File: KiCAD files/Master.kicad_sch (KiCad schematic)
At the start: 24 parts, among them SW1 EG1271A, SW2 EG1271A, SW3 EG1271A, SW4 EG1271A, U4 NUCLEO64-F446RE

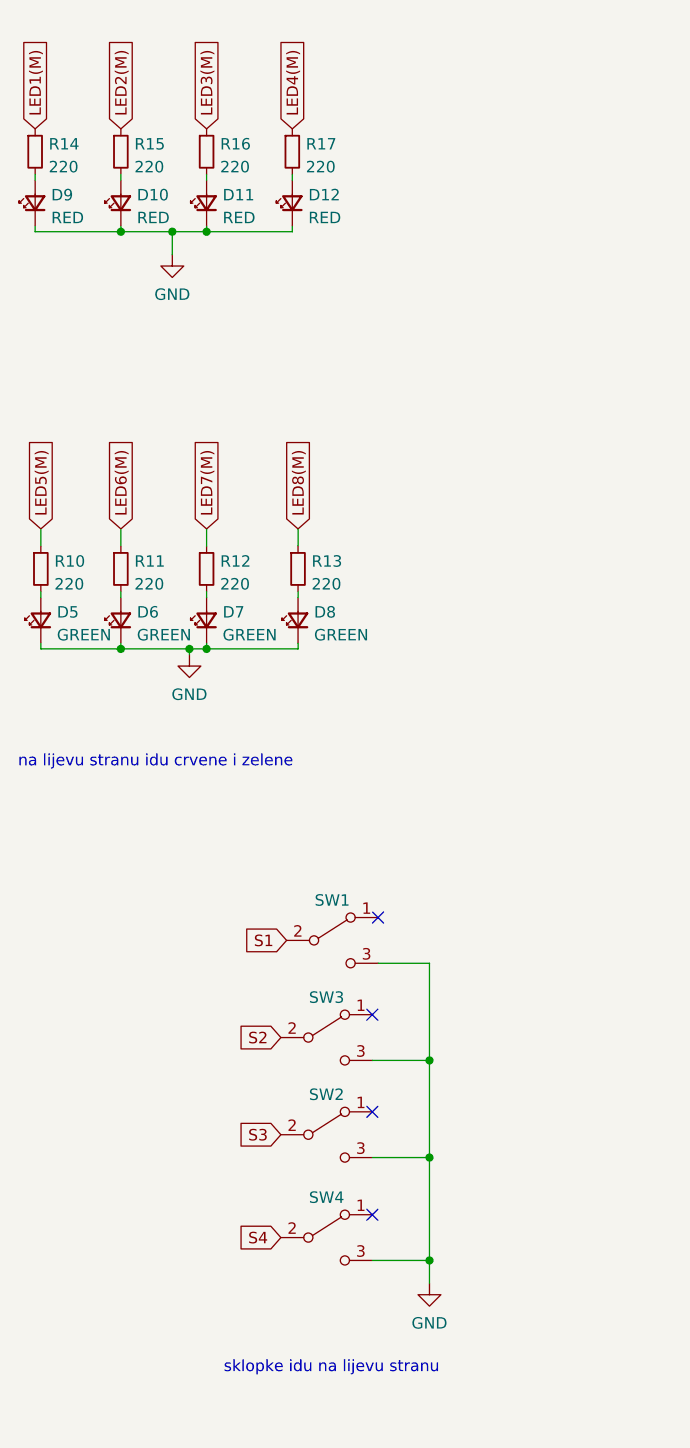
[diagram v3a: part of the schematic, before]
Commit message: update
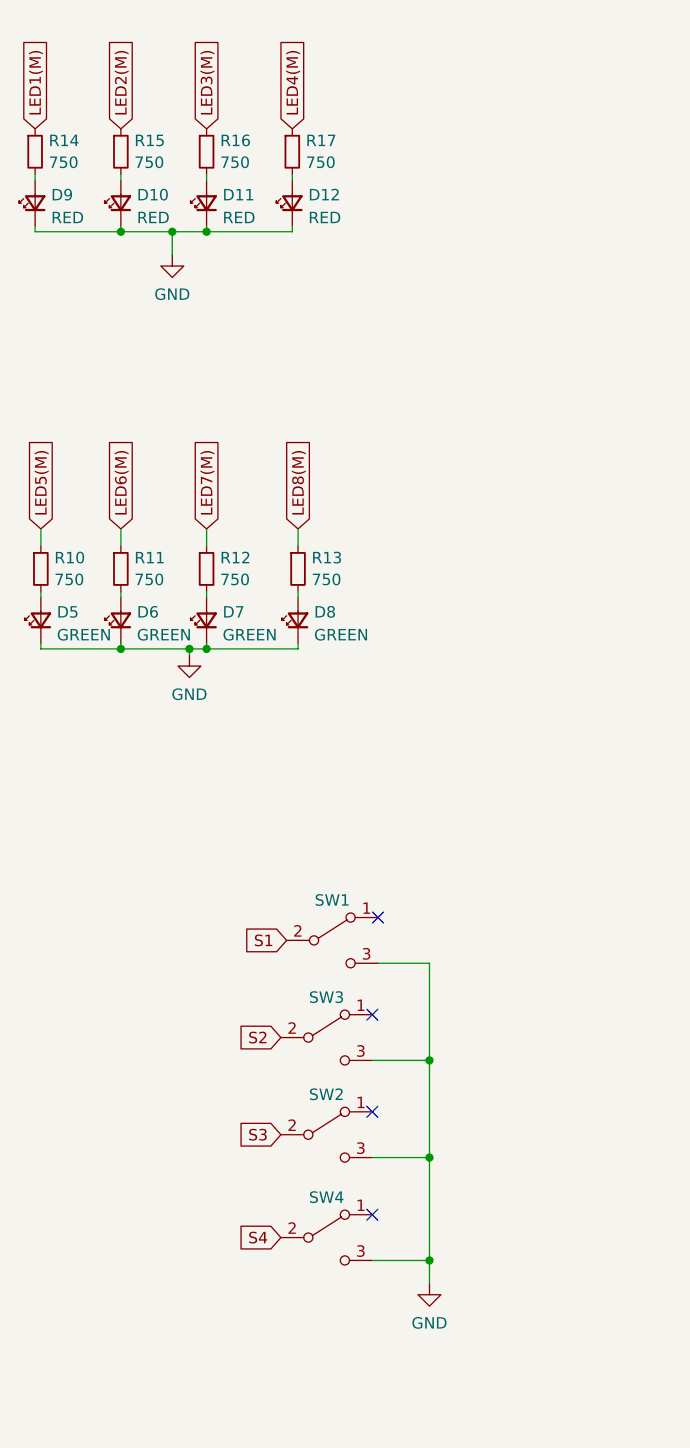
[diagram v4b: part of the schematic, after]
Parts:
- R10, R11, R12, R13, R14, R15, R16, R17: value 220 -> 750
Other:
- note removed: "na lijevu stranu idu crvene i zelene"
- note removed: "sklopke idu na lijevu stranu"
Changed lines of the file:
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@@
     (stroke (width 0) (type default))
-  )
-  (text "sklopke idu na lijevu stranu" (at 41.275 176.53 0)
-    (effects (font (size 1.27 1.27)) (justify left bottom))
   )
   (text "DAC MASTER" (at 106.045 175.895 0)
     (effects (font (size 1.27 1.27)) (justify left bottom))
   )
-  (text "na lijevu stranu idu crvene i zelene" (at 18.415 109.22 0)
-    (effects (font (size 1.27 1.27)) (justify left bottom))
-  )
   (global_label "S3" (shape input) (at 113.665 121.92 180) (fields_autoplaced)
     (effects (font (size 1.27 1.27)) (justify right))
@@
   (symbol (lib_id "Device:R_Small") (at 20.32 40.64 0) (unit 1)
     (in_bom yes) (on_board yes) (dnp no) (fields_autoplaced)
-    (property "Reference" "R14" (at 21.8186 39.8053 0)
-      (effects (font (size 1.27 1.27)) (justify left))
-    )
-    (property "Value" "220" (at 21.8186 42.3422 0)
+    (property "Reference" "R14" (at 21.8186 39.4279 0)
+      (effects (font (size 1.27 1.27)) (justify left))
+    )
+    (property "Value" "750" (at 21.8186 41.8521 0)
       (effects (font (size 1.27 1.27)) (justify left))
     )
@@
   (symbol (lib_id "Device:R_Small") (at 39.37 40.64 0) (unit 1)
     (in_bom yes) (on_board yes) (dnp no) (fields_autoplaced)
-    (property "Reference" "R16" (at 40.8686 39.8053 0)
-      (effects (font (size 1.27 1.27)) (justify left))
-    )
-    (property "Value" "220" (at 40.8686 42.3422 0)
+    (property "Reference" "R16" (at 40.8686 39.4279 0)
+      (effects (font (size 1.27 1.27)) (justify left))
+    )
+    (property "Value" "750" (at 40.8686 41.8521 0)
       (effects (font (size 1.27 1.27)) (justify left))
     )
@@
   (symbol (lib_id "Device:R_Small") (at 29.845 86.995 0) (unit 1)
     (in_bom yes) (on_board yes) (dnp no) (fields_autoplaced)
-    (property "Reference" "R11" (at 31.3436 86.1603 0)
-      (effects (font (size 1.27 1.27)) (justify left))
-    )
-    (property "Value" "220" (at 31.3436 88.6972 0)
+    (property "Reference" "R11" (at 31.3436 85.7829 0)
+      (effects (font (size 1.27 1.27)) (justify left))
+    )
+    (property "Value" "750" (at 31.3436 88.2071 0)
       (effects (font (size 1.27 1.27)) (justify left))
     )
@@
   (symbol (lib_id "Device:R_Small") (at 49.53 86.995 0) (unit 1)
     (in_bom yes) (on_board yes) (dnp no) (fields_autoplaced)
-    (property "Reference" "R13" (at 51.0286 86.1603 0)
-      (effects (font (size 1.27 1.27)) (justify left))
-    )
-    (property "Value" "220" (at 51.0286 88.6972 0)
+    (property "Reference" "R13" (at 51.0286 85.7829 0)
+      (effects (font (size 1.27 1.27)) (justify left))
+    )
+    (property "Value" "750" (at 51.0286 88.2071 0)
       (effects (font (size 1.27 1.27)) (justify left))
     )
@@
   (symbol (lib_id "Device:R_Small") (at 29.845 40.64 0) (unit 1)
     (in_bom yes) (on_board yes) (dnp no) (fields_autoplaced)
-    (property "Reference" "R15" (at 31.3436 39.8053 0)
-      (effects (font (size 1.27 1.27)) (justify left))
-    )
-    (property "Value" "220" (at 31.3436 42.3422 0)
+    (property "Reference" "R15" (at 31.3436 39.4279 0)
+      (effects (font (size 1.27 1.27)) (justify left))
+    )
+    (property "Value" "750" (at 31.3436 41.8521 0)
       (effects (font (size 1.27 1.27)) (justify left))
     )
@@
   (symbol (lib_id "Device:R_Small") (at 20.955 86.995 0) (unit 1)
     (in_bom yes) (on_board yes) (dnp no) (fields_autoplaced)
-    (property "Reference" "R10" (at 22.4536 86.1603 0)
-      (effects (font (size 1.27 1.27)) (justify left))
-    )
-    (property "Value" "220" (at 22.4536 88.6972 0)
+    (property "Reference" "R10" (at 22.4536 85.7829 0)
+      (effects (font (size 1.27 1.27)) (justify left))
+    )
+    (property "Value" "750" (at 22.4536 88.2071 0)
       (effects (font (size 1.27 1.27)) (justify left))
     )
@@
   (symbol (lib_id "Device:R_Small") (at 48.895 40.64 0) (unit 1)
     (in_bom yes) (on_board yes) (dnp no) (fields_autoplaced)
-    (property "Reference" "R17" (at 50.3936 39.8053 0)
-      (effects (font (size 1.27 1.27)) (justify left))
-    )
-    (property "Value" "220" (at 50.3936 42.3422 0)
+    (property "Reference" "R17" (at 50.3936 39.4279 0)
+      (effects (font (size 1.27 1.27)) (justify left))
+    )
+    (property "Value" "750" (at 50.3936 41.8521 0)
       (effects (font (size 1.27 1.27)) (justify left))
     )
@@
   (symbol (lib_id "Device:R_Small") (at 39.37 86.995 0) (unit 1)
     (in_bom yes) (on_board yes) (dnp no) (fields_autoplaced)
-    (property "Reference" "R12" (at 40.8686 86.1603 0)
-      (effects (font (size 1.27 1.27)) (justify left))
-    )
-    (property "Value" "220" (at 40.8686 88.6972 0)
-      (effects (font (size 1.27 1.27)) (justify left))
-    )
+    (property "Reference" "R12" (at 40.8686 85.7829 0)
+      (effects (font (size 1.27 1.27)) (justify left))
+    )
+    (property "Value" "750" (at 40.8686 88.2071 0)
+      (effects (font (size 1.27 1.27)) (justify left))
+    )

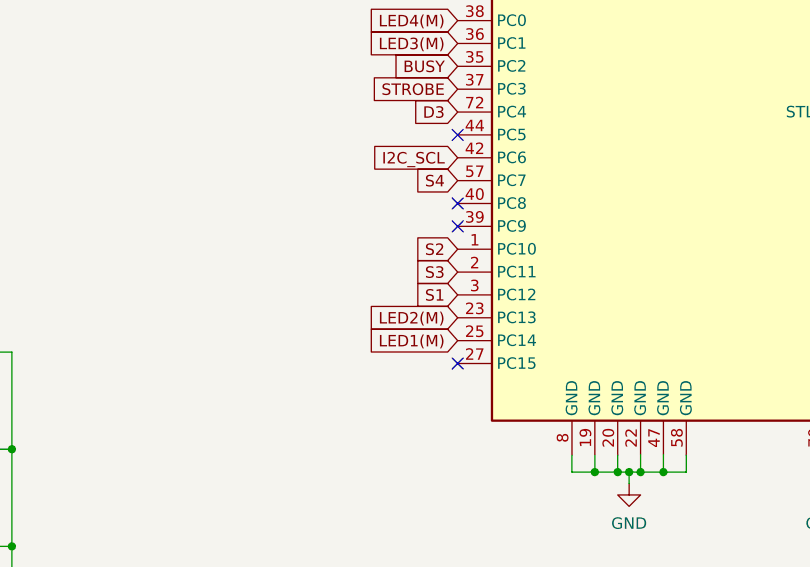
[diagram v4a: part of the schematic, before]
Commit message: update
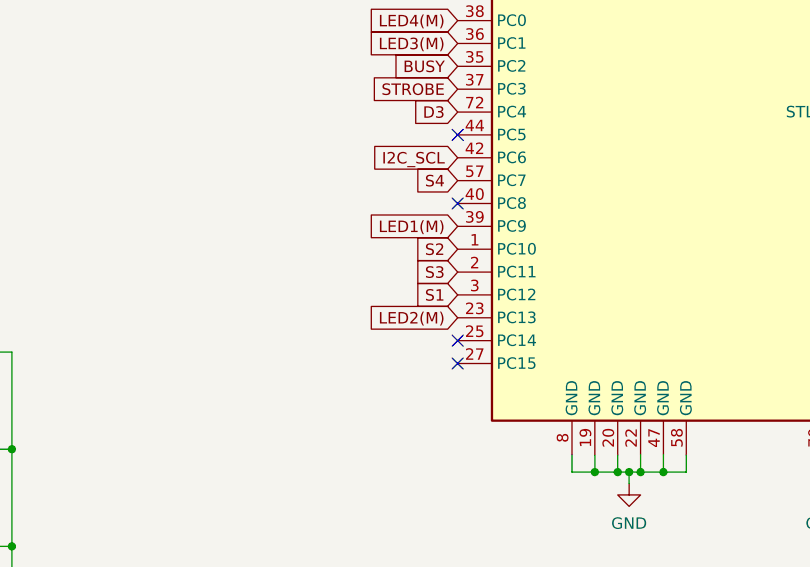
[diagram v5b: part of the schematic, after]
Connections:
- net LED1(M): now also U4.39 (PC9); no longer U4.25 (PC14)
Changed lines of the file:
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@@
   (no_connect (at 57.785 136.525))
   (no_connect (at 113.665 53.34))
-  (no_connect (at 113.665 116.84))
   (no_connect (at 113.665 106.68))
   (no_connect (at 57.785 158.75))
@@
   (no_connect (at 113.665 83.82))
   (no_connect (at 169.545 88.9))
+  (no_connect (at 113.665 129.54))
   (no_connect (at 57.785 147.32))
   (no_connect (at 113.665 55.88))
@@
     )
   )
-  (global_label "LED1(M)" (shape input) (at 113.665 129.54 180) (fields_autoplaced)
-    (effects (font (size 1.27 1.27)) (justify right))
-    (property "Intersheetrefs" "${INTERSHEET_REFS}" (at 102.8784 129.54 0)
-      (effects (font (size 1.27 1.27)) (justify right) hide)
-    )
+  (global_label "LED1(M)" (shape input) (at 113.665 116.84 180) (fields_autoplaced)
+    (effects (font (size 1.27 1.27)) (justify right))
+    (property "Intersheetrefs" "${INTERSHEET_REFS}" (at 102.8784 116.84 0)
+      (effects (font (size 1.27 1.27)) (justify right) hide)
+    )

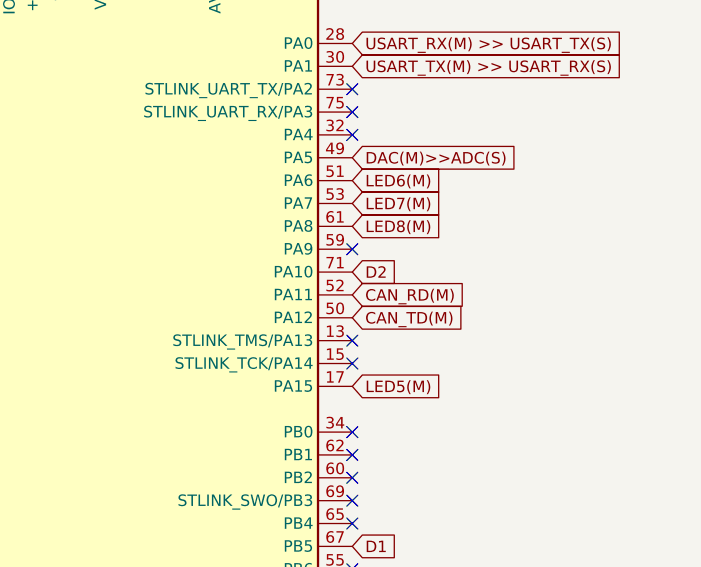
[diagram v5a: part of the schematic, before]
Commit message: update
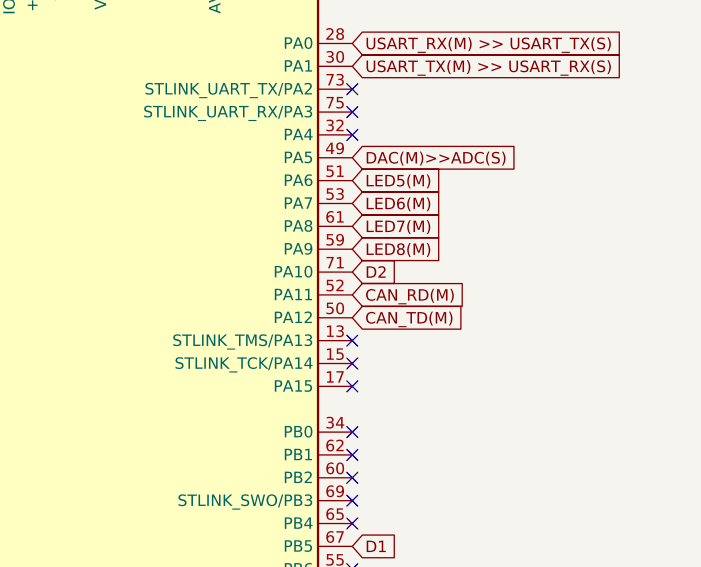
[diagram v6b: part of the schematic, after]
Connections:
- net LED5(M): now also U4.51 (PA6); no longer U4.17 (PA15)
- net LED6(M): now also U4.53 (PA7); no longer U4.51 (PA6)
- net LED7(M): now also U4.61 (PA8); no longer U4.53 (PA7)
- net LED8(M): now also U4.59 (PA9); no longer U4.61 (PA8)
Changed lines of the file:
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@@
   (no_connect (at 169.545 58.42))
   (no_connect (at 169.545 63.5))
+  (no_connect (at 169.545 91.44))
   (no_connect (at 128.905 40.64))
   (no_connect (at 113.665 88.9))
@@
   (no_connect (at 169.545 96.52))
   (no_connect (at 113.665 132.08))
-  (no_connect (at 169.545 76.2))
   (no_connect (at 126.365 40.64))
   (no_connect (at 169.545 86.36))
@@
     )
   )
-  (global_label "LED5(M)" (shape input) (at 169.545 91.44 0) (fields_autoplaced)
-    (effects (font (size 1.27 1.27)) (justify left))
-    (property "Intersheetrefs" "${INTERSHEET_REFS}" (at 180.3316 91.44 0)
+  (global_label "LED5(M)" (shape input) (at 169.545 68.58 0) (fields_autoplaced)
+    (effects (font (size 1.27 1.27)) (justify left))
+    (property "Intersheetrefs" "${INTERSHEET_REFS}" (at 180.3316 68.58 0)
       (effects (font (size 1.27 1.27)) (justify left) hide)
     )
@@
     )
   )
-  (global_label "LED8(M)" (shape input) (at 169.545 73.66 0) (fields_autoplaced)
+  (global_label "LED8(M)" (shape input) (at 169.545 76.2 0) (fields_autoplaced)
+    (effects (font (size 1.27 1.27)) (justify left))
+    (property "Intersheetrefs" "${INTERSHEET_REFS}" (at 180.3316 76.2 0)
+      (effects (font (size 1.27 1.27)) (justify left) hide)
+    )
+  )
+  (global_label "LED6(M)" (shape input) (at 169.545 71.12 0) (fields_autoplaced)
+    (effects (font (size 1.27 1.27)) (justify left))
+    (property "Intersheetrefs" "${INTERSHEET_REFS}" (at 180.3316 71.12 0)
+      (effects (font (size 1.27 1.27)) (justify left) hide)
+    )
+  )
+  (global_label "DAC(M)>>ADC(S)" (shape input) (at 107.95 172.085 0) (fields_autoplaced)
+    (effects (font (size 1.27 1.27)) (justify left))
+    (property "Intersheetrefs" "${INTERSHEET_REFS}" (at 127.3849 172.085 0)
+      (effects (font (size 1.27 1.27)) (justify left) hide)
+    )
+  )
+  (global_label "S1" (shape input) (at 48.26 128.27 180) (fields_autoplaced)
+    (effects (font (size 1.27 1.27)) (justify right))
+    (property "Intersheetrefs" "${INTERSHEET_REFS}" (at 42.8558 128.27 0)
+      (effects (font (size 1.27 1.27)) (justify right) hide)
+    )
+  )
+  (global_label "LED5(M)" (shape input) (at 20.955 82.55 90) (fields_autoplaced)
+    (effects (font (size 1.27 1.27)) (justify left))
+    (property "Intersheetrefs" "${INTERSHEET_REFS}" (at 20.955 71.7634 90)
+      (effects (font (size 1.27 1.27)) (justify left) hide)
+    )
+  )
+  (global_label "BUSY" (shape input) (at 113.665 99.06 180) (fields_autoplaced)
+    (effects (font (size 1.27 1.27)) (justify right))
+    (property "Intersheetrefs" "${INTERSHEET_REFS}" (at 105.7812 99.06 0)
+      (effects (font (size 1.27 1.27)) (justify right) hide)
+    )
+  )
+  (global_label "LED1(M)" (shape input) (at 20.32 38.1 90) (fields_autoplaced)
+    (effects (font (size 1.27 1.27)) (justify left))
+    (property "Intersheetrefs" "${INTERSHEET_REFS}" (at 20.32 27.3134 90)
+      (effects (font (size 1.27 1.27)) (justify left) hide)
+    )
+  )
+  (global_label "LED4(M)" (shape input) (at 113.665 93.98 180) (fields_autoplaced)
+    (effects (font (size 1.27 1.27)) (justify right))
+    (property "Intersheetrefs" "${INTERSHEET_REFS}" (at 102.8784 93.98 0)
+      (effects (font (size 1.27 1.27)) (justify right) hide)
+    )
+  )
+  (global_label "S2" (shape input) (at 47.625 139.065 180) (fields_autoplaced)
+    (effects (font (size 1.27 1.27)) (justify right))
+    (property "Intersheetrefs" "${INTERSHEET_REFS}" (at 42.2208 139.065 0)
+      (effects (font (size 1.27 1.27)) (justify right) hide)
+    )
+  )
+  (global_label "I2C_SCL" (shape input) (at 113.665 109.22 180) (fields_autoplaced)
+    (effects (font (size 1.27 1.27)) (justify right))
+    (property "Intersheetrefs" "${INTERSHEET_REFS}" (at 103.1203 109.22 0)
+      (effects (font (size 1.27 1.27)) (justify right) hide)
+    )
+  )
+  (global_label "LED7(M)" (shape input) (at 169.545 73.66 0) (fields_autoplaced)
     (effects (font (size 1.27 1.27)) (justify left))
     (property "Intersheetrefs" "${INTERSHEET_REFS}" (at 180.3316 73.66 0)
       (effects (font (size 1.27 1.27)) (justify left) hide)
     )
-  )
-  (global_label "LED6(M)" (shape input) (at 169.545 68.58 0) (fields_autoplaced)
-    (effects (font (size 1.27 1.27)) (justify left))
-    (property "Intersheetrefs" "${INTERSHEET_REFS}" (at 180.3316 68.58 0)
-      (effects (font (size 1.27 1.27)) (justify left) hide)
-    )
-  )
-  (global_label "DAC(M)>>ADC(S)" (shape input) (at 107.95 172.085 0) (fields_autoplaced)
-    (effects (font (size 1.27 1.27)) (justify left))
-    (property "Intersheetrefs" "${INTERSHEET_REFS}" (at 127.3849 172.085 0)
-      (effects (font (size 1.27 1.27)) (justify left) hide)
-    )
-  )
-  (global_label "S1" (shape input) (at 48.26 128.27 180) (fields_autoplaced)
-    (effects (font (size 1.27 1.27)) (justify right))
-    (property "Intersheetrefs" "${INTERSHEET_REFS}" (at 42.8558 128.27 0)
-      (effects (font (size 1.27 1.27)) (justify right) hide)
-    )
-  )
-  (global_label "LED5(M)" (shape input) (at 20.955 82.55 90) (fields_autoplaced)
-    (effects (font (size 1.27 1.27)) (justify left))
-    (property "Intersheetrefs" "${INTERSHEET_REFS}" (at 20.955 71.7634 90)
-      (effects (font (size 1.27 1.27)) (justify left) hide)
-    )
-  )
-  (global_label "BUSY" (shape input) (at 113.665 99.06 180) (fields_autoplaced)
-    (effects (font (size 1.27 1.27)) (justify right))
-    (property "Intersheetrefs" "${INTERSHEET_REFS}" (at 105.7812 99.06 0)
-      (effects (font (size 1.27 1.27)) (justify right) hide)
-    )
-  )
-  (global_label "LED1(M)" (shape input) (at 20.32 38.1 90) (fields_autoplaced)
-    (effects (font (size 1.27 1.27)) (justify left))
-    (property "Intersheetrefs" "${INTERSHEET_REFS}" (at 20.32 27.3134 90)
-      (effects (font (size 1.27 1.27)) (justify left) hide)
-    )
-  )
-  (global_label "LED4(M)" (shape input) (at 113.665 93.98 180) (fields_autoplaced)
-    (effects (font (size 1.27 1.27)) (justify right))
-    (property "Intersheetrefs" "${INTERSHEET_REFS}" (at 102.8784 93.98 0)
-      (effects (font (size 1.27 1.27)) (justify right) hide)
-    )
-  )
-  (global_label "S2" (shape input) (at 47.625 139.065 180) (fields_autoplaced)
-    (effects (font (size 1.27 1.27)) (justify right))
-    (property "Intersheetrefs" "${INTERSHEET_REFS}" (at 42.2208 139.065 0)
-      (effects (font (size 1.27 1.27)) (justify right) hide)
-    )
-  )
-  (global_label "I2C_SCL" (shape input) (at 113.665 109.22 180) (fields_autoplaced)
-    (effects (font (size 1.27 1.27)) (justify right))
-    (property "Intersheetrefs" "${INTERSHEET_REFS}" (at 103.1203 109.22 0)
-      (effects (font (size 1.27 1.27)) (justify right) hide)
-    )
-  )
-  (global_label "LED7(M)" (shape input) (at 169.545 71.12 0) (fields_autoplaced)
-    (effects (font (size 1.27 1.27)) (justify left))
-    (property "Intersheetrefs" "${INTERSHEET_REFS}" (at 180.3316 71.12 0)
-      (effects (font (size 1.27 1.27)) (justify left) hide)
-    )
